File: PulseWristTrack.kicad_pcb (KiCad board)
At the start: 4 copper layers, 36 x 36 mm, 18 parts, among them J1 LiPo, Q1 BSS138, Q2 BSS138, SW1 JS202011MQN, U1 XIAO nRF52840 Sense, U2 MAX30102, U3 AP2112K-1.8

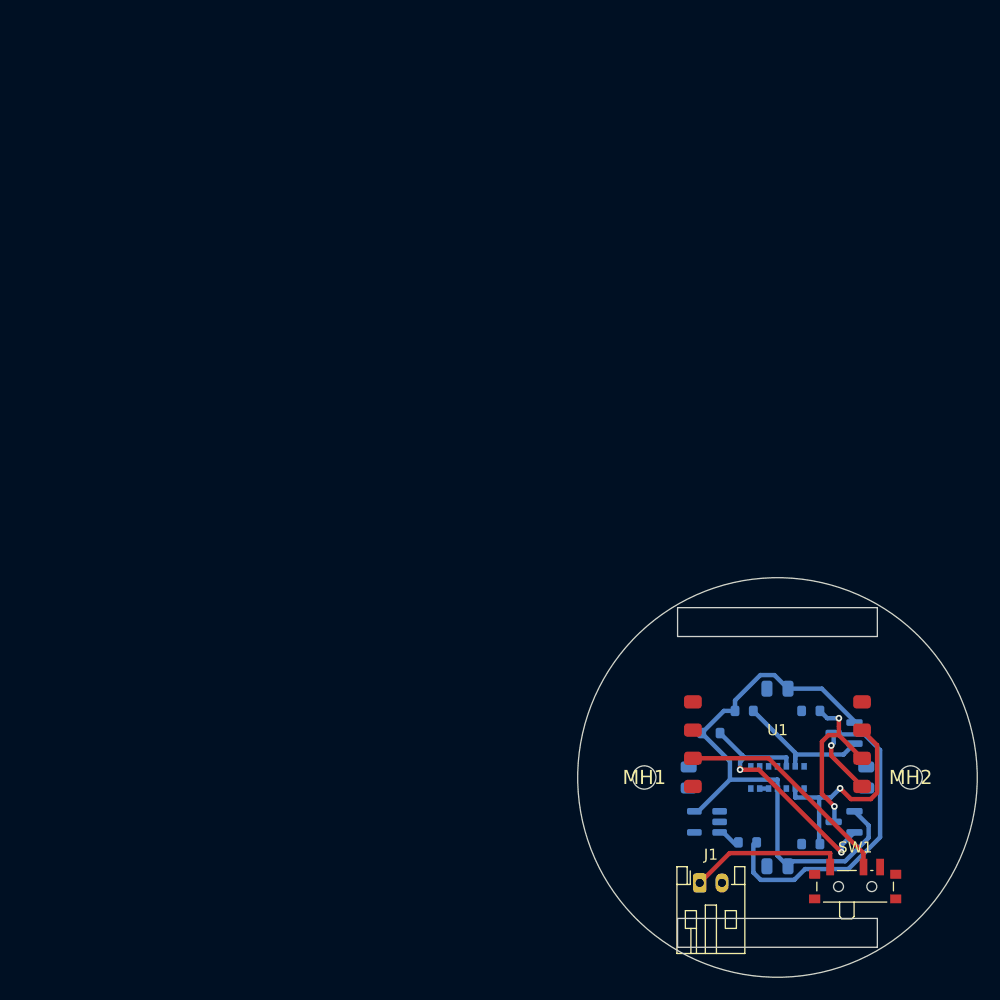
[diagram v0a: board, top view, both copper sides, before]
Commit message: auto-backup 2026-07-24 19:26:27
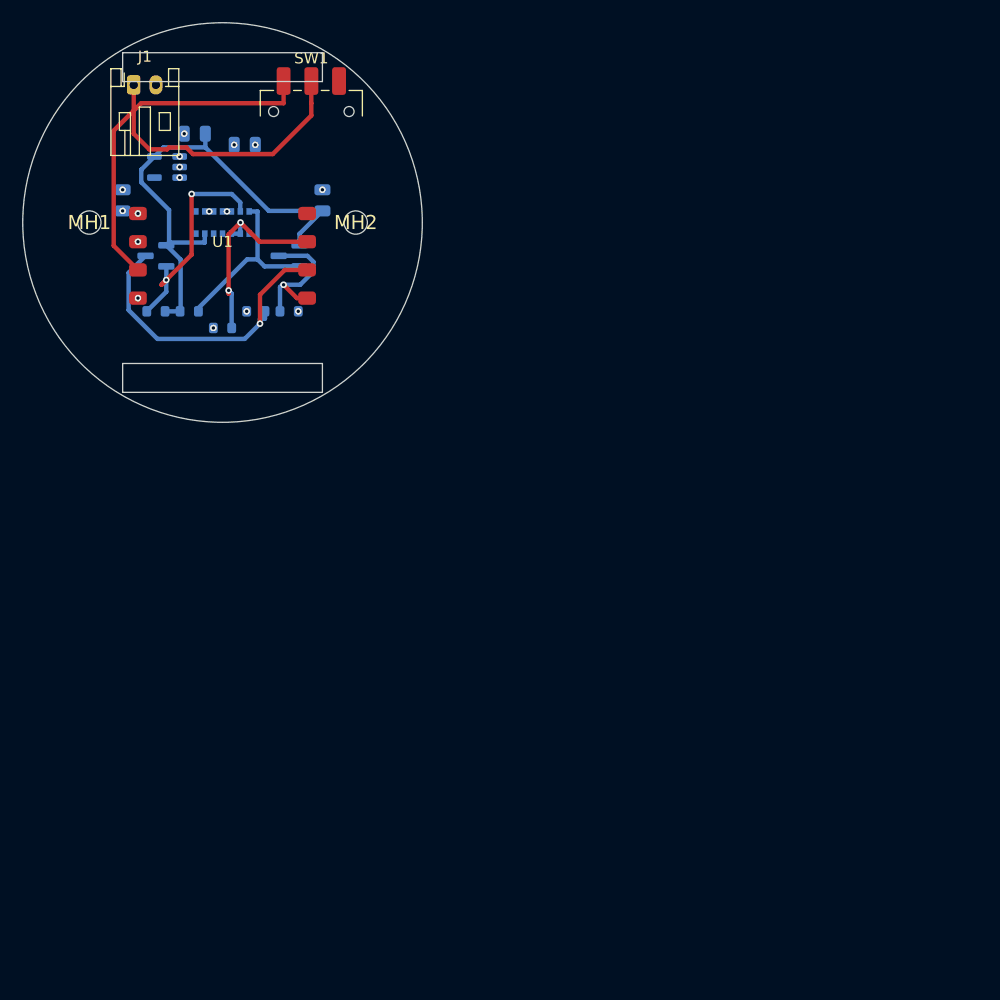
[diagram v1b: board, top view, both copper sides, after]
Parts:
- J1: value LiPo -> BATT_JST_PH
- SW1: value JS202011MQN -> JS102011SAQN; footprint Button_Switch_SMD:SW_SPDT_PCM12 -> Button_Switch_SMD:SW_SPDT_CK_JS102011SAQN
- U1: value XIAO nRF52840 Sense -> XIAO_nRF52840_Sense
- moved J1 88.2 mm to (-8.00, -12.4)
- moved SW1 85.0 mm to (8.00, -10.0)
- moved C2 84.3 mm to (-2.50, -8.00)
- moved Q1 80.3 mm to (-6.00, 3.00)
- moved C3 79.9 mm to (2.00, -7.00), turned to 0 degrees
- moved U3 76.5 mm to (-5.00, -5.00)
- moved C1 72.8 mm to (-9.00, -2.00)
- moved MH1 70.7 mm to (-12.0, 0.00)
- moved MH2 70.7 mm to (12.0, 0.00)
- moved U2 70.7 mm to (0.00, 0.00)
- moved R5 70.5 mm to (0.00, 9.50)
- moved U1 66.6 mm to (0.00, 3.00)
- moved Q2 65.9 mm to (6.00, 3.00)
- moved R4 63.2 mm to (6.00, 8.00), turned to 0 degrees
- moved R1 62.8 mm to (-6.00, 8.00), turned to 0 degrees
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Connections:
- J1 pad 1: BAT_RAW -> BAT+
- SW1 pad 1: BAT_RAW -> BAT_SW
- SW1 pad 2: BAT_SW -> BAT+
- U2 pad 1: (no net) -> SCL_1V8
- U2 pad 11: +1V8 -> GND
- U2 pad 12: GND -> INT
- U2 pad 2: SCL_1V8 -> SDA_1V8
- U2 pad 3: SDA_1V8 -> GND
- U2 pad 5: (no net) -> +3V3
- U2 pad 6: (no net) -> +3V3
- U2 pad 9: +3V3 -> +1V8
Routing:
- net BAT+: track 0.00 -> 25.8 mm
- net SCL_3V3: track 34.5 -> 12.6 mm
- net BAT_RAW: track 14.1 -> 0.00 mm
- net SDA_3V3: track 16.1 -> 28.3 mm, vias 2 -> 1
- net BAT_SW: track 20.2 -> 31.8 mm
- net +1V8: track 51.3 -> 44.5 mm
- net SCL_1V8: track 12.3 -> 16.6 mm
- net SDA_1V8: track 25.4 -> 21.4 mm
- net +3V3: track 2.28 -> 0.40 mm, vias 0 -> 9
- net GND: track 0.00 -> 0.40 mm, vias 0 -> 8
- net INT: track 19.6 -> 19.7 mm, vias 1 -> 2
